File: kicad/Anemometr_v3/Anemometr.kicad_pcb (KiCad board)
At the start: 2 copper layers, 45 x 45 mm, 150 parts, among them J1 TxD, J10 +Z1, J11 +Z2, J12 +Z3, J13 +Z4, J14 -Z1, J15 -Z2, J16 -Z3, J17 -Z4, J18 1 TxD+, J19 2 TxD-, J2 RxD, J20 3 RxD+, J21 4-5, J22 6 RxD-, J23 7-8, J24 Conn_01x01_Female, J25 Conn_01x01_Female, J3 SCL, J4 SDA, J5 RST, J6 +EXT, J7 -EXT, J8 SWD, J9 SWC, Q1 5N10, U1 STM32F103C8Tx, U2 TS5A3166DBVR, U3 TS5A3166DBVR, U4 LMR14206, U6 NCP1117-3.3, U8 TLV3201DBV, U9 MCP1703-3.3, Y1 CSTCE8M00G52A-R0, Y2 ECS-250-20-33

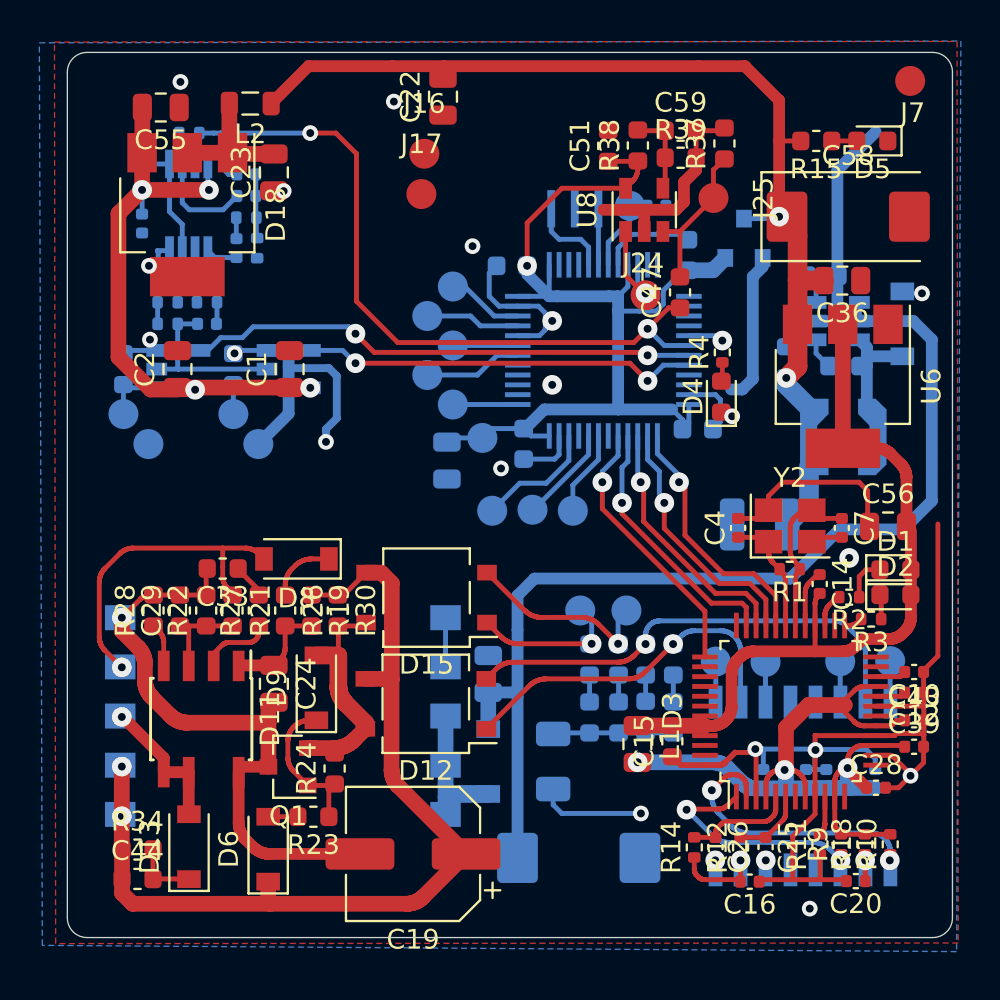
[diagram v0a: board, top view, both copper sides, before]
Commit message: изменено:      kicad/Anemometr_v3/Anemometr-cache.lib 	изменено:      kicad/Anemometr_v3/Anemometr.kicad_pcb 	изменено:      kicad/Anemometr_v3/Anemometr.kicad_pcb-bak 	изменено:      kicad/Anemometr_v3/Anemometr.sch 	изменено:      kicad/Anemometr_v3/Anemometr.sch-bak 	новый файл:    stm32cubeide/Anemometer/Debug/Core/Src/dhcp.d 	новый файл:    stm32cubeide/Anemometer/Debug/Core/Src/dhcp.o 	новый файл:    stm32cubeide/Anemometer/Debug/Core/Src/dhcp.su 	новый файл:    stm32cubeide/Anemometer/Debug/Core/Src/dns.d 	новый файл:    stm32cubeide/Anemometer/Debug/Core/Src/dns.o 	новый файл:    stm32cubeide/Anemometer/Debug/Core/Src/dns.su 	новый файл:    stm32cubeide/Anemometer/Debug/Core/Src/socket.d 	новый файл:    stm32cubeide/Anemometer/Debug/Core/Src/socket.o 	новый файл:    stm32cubeide/Anemometer/Debug/Core/Src/socket.su 	новый файл:    stm32cubeide/Anemometer/Debug/Core/Src/w5500.d 	новый файл:    stm32cubeide/Anemometer/Debug/Core/Src/w5500.o 	новый файл:    stm32cubeide/Anemometer/Debug/Core/Src/w5500.su 	новый файл:    stm32cubeide/Anemometer/Debug/Core/Src/wizchip_conf.d 	новый файл:    stm32cubeide/Anemometer/Debug/Core/Src/wizchip_conf.o 	новый файл:    stm32cubeide/Anemometer/Debug/Core/Src/wizchip_conf.su 	новый файл:    stm32cubeide/Anemometer/Debug/Drivers/STM32F1xx_HAL_Driver/Src/stm32f1xx_hal_i2c.d 	новый файл:    stm32cubeide/Anemometer/Debug/Drivers/STM32F1xx_HAL_Driver/Src/stm32f1xx_hal_i2c.o 	новый файл:    stm32cubeide/Anemometer/Debug/Drivers/STM32F1xx_HAL_Driver/Src/stm32f1xx_hal_i2c.su 	новый файл:    stm32cubeide/Anemometer/Drivers/STM32F1xx_HAL_Driver/Inc/stm32f1xx_hal_iwdg.h 	новый файл:    stm32cubeide/Anemometer/Drivers/STM32F1xx_HAL_Driver/Inc/stm32f1xx_hal_spi.h 	новый файл:    stm32cubeide/Anemometer/Drivers/STM32F1xx_HAL_Driver/Src/stm32f1xx_hal_iwdg.c 	новый файл:    stm32cubeide/Anemometer/Drivers/STM32F1xx_HAL_Driver/Src/stm32f1xx_hal_spi.c 	новый файл:    stm32cubeide/Anemometer/Release/Anemometer.hex 	новый файл:    stm32cubeide/A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
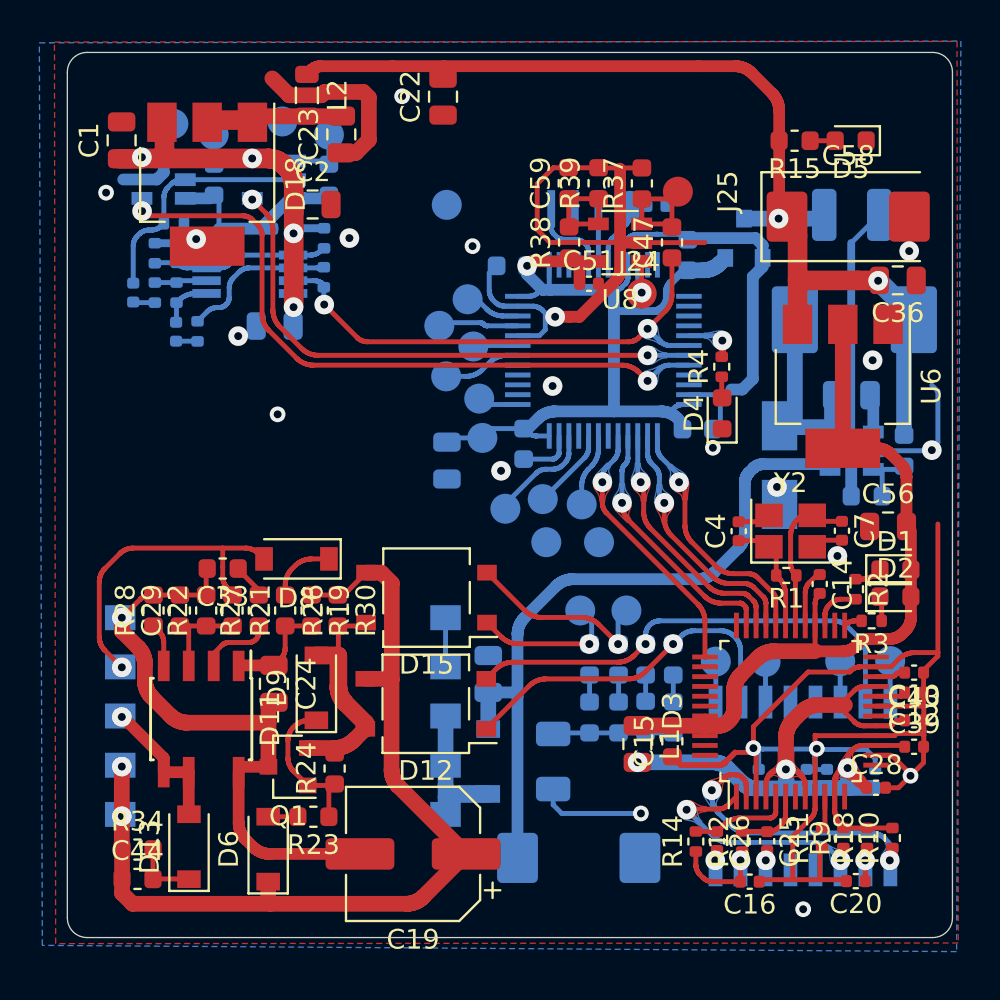
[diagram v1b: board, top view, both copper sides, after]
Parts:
- removed C40, C41: 390p, Capacitor_SMD:C_0402_1005Metric
- removed R31: 1.3k, Resistor_SMD:R_0402_1005Metric
- C51: footprint Capacitor_SMD:C_0603_1608Metric -> Capacitor_SMD:C_0402_1005Metric
- C53: footprint Capacitor_SMD:C_0603_1608Metric -> Capacitor_SMD:C_0805_2012Metric
- C55, J16, J17, J7: moved to B.Cu
- D13, D8: value MBR0540 -> F7
- D16: value MBR0540 -> SS34
- D17: value MBR0540 -> SS56; footprint Diode_SMD:D_SOD-123 -> Diode_SMD:D_SMA
- L5: value CoilCraft HLPS4018-472MR -> 15uH; footprint Inductor_SMD:L_Coilcraft_LPS4018 -> Inductor_SMD:L_Abracon_ASPI-0630LR
- R17: value 110k -> 100k
- moved J7 29.9 mm to (43.4, 84.9)
- moved J16 21.7 mm to (46.0, 84.9)
- moved J15 17.8 mm to (29.9, 63.5), turned to 180 degrees
- moved J10 17.6 mm to (32.3, 64.2), turned to 180 degrees
- moved J14 16.8 mm to (24.4, 63.6), turned to 180 degrees
- moved C54 16.4 mm to (58.9, 68.3), turned to 180 degrees
- moved C1 14.4 mm to (21.8, 64.5)
- moved J11 14.2 mm to (26.4, 64.2), turned to 180 degrees
- moved R5 14.2 mm to (32.3, 66.5), turned to 90 degrees
- moved C55 12.5 mm to (29.5, 73.9), turned to 0 degrees
- moved U3 11.5 mm to (23.9, 66.5), turned to 180 degrees
- moved R41 11.4 mm to (59.6, 82.6), turned to 180 degrees
- moved C2 10.8 mm to (31.5, 67.7), turned to 0 degrees
- moved U2 10.8 mm to (29.5, 66.5), turned to 180 degrees
- moved R33 10.0 mm to (32.0, 71.4), turned to 270 degrees
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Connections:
- net Net-(C22-Pad2) renamed /5.6-6v
- net Net-(C3-Pad2) renamed /Rst
- net Net-(J1-Pad1) renamed /TxD
- net Net-(J10-Pad1) renamed /+Z1
- net Net-(J11-Pad1) renamed /+Z2
- net Net-(J12-Pad1) renamed /+Z3
- net Net-(J13-Pad1) renamed /+Z4
- net Net-(J2-Pad1) renamed /RxD
- net Net-(J3-Pad1) renamed /SCL
- net Net-(J4-Pad1) renamed /SDA
- net Net-(J8-Pad1) renamed /SWD
- net Net-(J9-Pad1) renamed /SWC
- D3 pad 23: (no net) -> GND
- D7 pad 6: Net-(C41-Pad2) -> Net-(D7-Pad6)
- R29 pad 1: Net-(C40-Pad1) -> Net-(D7-Pad6)
- R33 pad 1: Net-(C41-Pad2) -> Net-(D7-Pad6)
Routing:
- net GND: track 146.0 -> 190.4 mm, vias 19 -> 21
- net /12-16v: track 53.5 -> 37.7 mm
- net Z2: track 20.2 -> 34.9 mm
- net Analog: track 40.8 -> 26.5 mm
- net +5VA: track 30.5 -> 21.4 mm
- net Net-(D7-Pad6): track 0.00 -> 8.04 mm
- net +3V3: track 50.5 -> 43.3 mm
- net Net-(C41-Pad2): track 6.82 -> 0.00 mm
- net Net-(C18-Pad2): track 8.93 -> 12.5 mm
- net Net-(C40-Pad1): track 3.27 -> 0.00 mm
- net /5.6-6v: track 57.4 -> 54.4 mm
- net Z1: track 26.0 -> 28.3 mm
- net SensorInput: track 5.28 -> 3.13 mm
- net Net-(R41-Pad1): track 4.97 -> 3.00 mm
- net Net-(C59-Pad1): track 4.37 -> 5.80 mm
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
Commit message: изменено:      kicad/Anemometr_v3/Anemometr-cache.lib 	изменено:      kicad/Anemometr_v3/Anemometr.kicad_pcb 	изменено:      kicad/Anemometr_v3/Anemometr.kicad_pcb-bak 	изменено:      kicad/Anemometr_v3/Anemometr.pro 	изменено:      kicad/Anemometr_v3/Anemometr.sch 	изменено:      kicad/Anemometr_v3/Anemometr.sch-bak 	изменено:      kicad/Anemometr_v3/fp-info-cache
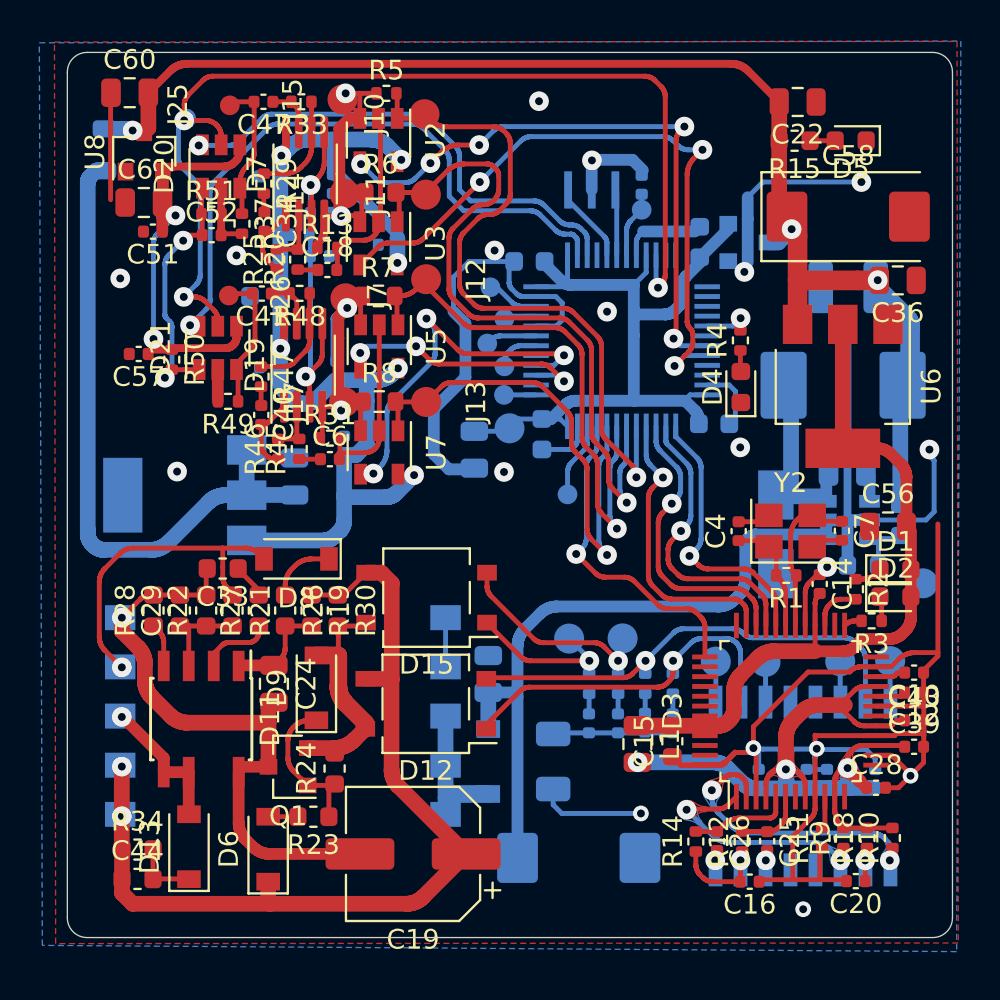
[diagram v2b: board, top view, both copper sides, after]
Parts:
- removed R38: 100k, Resistor_SMD:R_0603_1608Metric
- removed R39: 3k, Resistor_SMD:R_0603_1608Metric
- added C32: 0.1uF, Capacitor_SMD:C_0402_1005Metric, B.Cu at (29.2, 66.3)
- added C40: 100nF, Capacitor_SMD:C_0402_1005Metric, F.Cu at (28.9, 78.4)
- added C41: 1,5nF, Capacitor_SMD:C_0402_1005Metric, F.Cu at (28.9, 72.3)
- added C5: 0.1uF, Capacitor_SMD:C_0402_1005Metric, B.Cu at (33.1, 80.0)
- added C52: 0.1uF, Capacitor_SMD:C_0402_1005Metric, F.Cu at (26.3, 69.3)
- added C57: 0.1uF, Capacitor_SMD:C_0402_1005Metric, F.Cu at (22.6, 75.3)
- added C6: 10nF, Capacitor_SMD:C_0402_1005Metric, F.Cu at (32.4, 80.7)
- added C60: 10uF, Capacitor_SMD:C_0805_2012Metric, F.Cu at (22.2, 62.0)
- added C61: 10uF, Capacitor_SMD:C_0805_2012Metric, F.Cu at (22.9, 67.6)
- added D19: MAX4477, Package_SO:MSOP-8_3x3mm_P0.65mm, F.Cu at (31.0, 75.9)
- added D20: TLV3501, Package_TO_SOT_SMD:SOT-23-6, F.Cu at (26.8, 65.8)
- added D21: TLV3501, Package_TO_SOT_SMD:SOT-23-6, F.Cu at (26.6, 75.0)
- added J26: Conn_01x01_Female, My-library:ConnMini, F.Cu at (27.2, 72.4)
- added R31: 20k, Resistor_SMD:R_0402_1005Metric, F.Cu at (32.4, 79.6)
- added R45: 1k, Resistor_SMD:R_0402_1005Metric, F.Cu at (30.8, 80.2)
- added R46: 100k, Resistor_SMD:R_0402_1005Metric, F.Cu at (29.7, 80.2)
- added R47: 5.1k, Resistor_SMD:R_0402_1005Metric, F.Cu at (28.9, 76.5)
- added R48: 100k, Resistor_SMD:R_0402_1005Metric, F.Cu at (30.8, 72.2)
- added R49: 10k, Resistor_SMD:R_0402_1005Metric, F.Cu at (27.2, 77.7)
- added R50: 100k, Resistor_SMD:R_0402_1005Metric, F.Cu at (24.3, 75.6)
- added R51: 3k, Resistor_SMD:R_0402_1005Metric, F.Cu at (26.3, 68.2)
- added R7: 3k, Resistor_SMD:R_0603_1608Metric, F.Cu at (34.8, 72.4)
- added R8: 3k, Resistor_SMD:R_0603_1608Metric, F.Cu at (34.9, 77.8)
- added U5: TS5A3166DBVR, Package_TO_SOT_SMD:SOT-23-5, F.Cu at (34.9, 75.0)
- added U7: TS5A3166DBVR, Package_TO_SOT_SMD:SOT-23-5, F.Cu at (34.9, 80.3)
- C1, C2: footprint Capacitor_SMD:C_0805_2012Metric -> Capacitor_SMD:C_0402_1005Metric; moved to B.Cu
- C18, C34, D7, J10, J11, J12, J13, J14, J15, J17, J7, R13, R20, R29, R33, R6, U2, U3: moved to F.Cu
- C23, D18, L2: moved to B.Cu
- C42, C45, C46, C47, C48: footprint Capacitor_SMD:C_0603_1608Metric -> Capacitor_SMD:C_0402_1005Metric
- C55: footprint Capacitor_SMD:C_0805_2012Metric -> Capacitor_SMD:C_0603_1608Metric
- C59: footprint Capacitor_SMD:C_0603_1608Metric -> Capacitor_SMD:C_0402_1005Metric; moved to B.Cu
- J1, J2, J25, J3, J4, J5, J8, J9: footprint My-library:SMD-CONN -> My-library:ConnMini
- J24: footprint My-library:SMD-CONN -> My-library:ConnMini; moved to B.Cu
- R17: value 100k -> 110k
- R21: value 30k -> 43k
- R25: value 300k -> 100k; moved to F.Cu
- R32, R35, R36, R37, R40: footprint Resistor_SMD:R_0603_1608Metric -> Resistor_SMD:R_0402_1005Metric
- R5: footprint Resistor_SMD:R_0603_1608Metric -> Resistor_SMD:R_0402_1005Metric; moved to F.Cu
- U8: value TLV3201DBV -> MCP1703-3.3; footprint Package_TO_SOT_SMD:SOT-23-5 -> Package_TO_SOT_SMD:SOT-23
- moved J24 24.8 mm to (25.0, 63.4)
- moved U8 24.6 mm to (22.9, 65.1), turned to 90 degrees
- moved J25 23.2 mm to (27.3, 62.7), turned to 270 degrees
- moved C51 22.3 mm to (23.4, 69.1), turned to 180 degrees
- moved C47 22.0 mm to (29.0, 62.5), turned to 180 degrees
- moved R37 20.4 mm to (27.9, 68.7), turned to 270 degrees
- moved C22 18.0 mm to (56.1, 62.5), turned to 180 degrees
- moved C59 17.9 mm to (29.2, 76.0), turned to 180 degrees
- moved C23 17.6 mm to (30.6, 81.6), turned to 270 degrees
- moved J16 16.6 mm to (62.5, 87.0)
- moved J7 16.1 mm to (33.1, 72.5), turned to 90 degrees
- moved C1 16.0 mm to (32.7, 76.2)
- moved D18 15.9 mm to (25.0, 82.5), turned to 180 degrees
- moved J12 13.9 mm to (37.2, 71.5), turned to 90 degrees
- moved U3 11.4 mm to (34.8, 69.7), turned to 270 degrees
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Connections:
- net /SWC renamed /swc
- net /SWD renamed /swd
- net Net-(C21-Pad2) renamed a
- C47 pad 1: Analog -> Net-(C47-Pad1)
- C51 pad 1: +3V3 -> +3.3VP
- C59 pad 1: Net-(C59-Pad1) -> +5VA
- D7 pad 7: Analog -> Net-(C47-Pad1)
- J24 pad 1: SensorInput -> SInput
- R33 pad 2: Analog -> Net-(C47-Pad1)
- U1 pad 10: SensorInput -> SInput
- U1 pad 18: Analog -> (no net)
- U1 pad 2: (no net) -> Z3-4
- U1 pad 29: nrst -> /+Z1
- U1 pad 3: (no net) -> Z1-2
- U1 pad 30: (no net) -> /+Z2
- U1 pad 33: (no net) -> nrst
- U1 pad 39: (no net) -> Z3
- U1 pad 40: (no net) -> Z4
- U8 pad 1: SensorInput -> GND
- U8 pad 2: GND -> +3.3VP
- U8 pad 3: Net-(C47-Pad2) -> /5.6-6v
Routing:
- net SInput: track 0.00 -> 53.4 mm, vias 0 -> 3
- net +5VA: track 21.4 -> 54.4 mm, vias 4 -> 6
- net /+Z2: track 3.04 -> 35.9 mm, vias 0 -> 1
- net Z3-4: track 0.00 -> 32.2 mm, vias 0 -> 1
- net /+Z1: track 3.26 -> 35.0 mm, vias 0 -> 1
- net Net-(C23-Pad2): track 6.86 -> 33.4 mm
- net Analog: track 26.5 -> 0.00 mm, vias 2 -> 0
- net Z1-2: track 0.00 -> 24.9 mm, vias 0 -> 1
- net /+Z3: track 3.73 -> 28.1 mm, vias 0 -> 1
- net /+Z4: track 4.16 -> 25.9 mm, vias 0 -> 1
- net +3.3VP: track 0.00 -> 21.4 mm, vias 0 -> 2
- net Z4: track 0.00 -> 19.2 mm, vias 0 -> 3
- net Z3: track 0.00 -> 13.5 mm, vias 0 -> 3
- net Net-(C52-Pad1): track 0.00 -> 13.2 mm, vias 0 -> 2
- net /5.6-6v: track 54.4 -> 67.2 mm, vias 2 -> 3
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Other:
- net class Default: via_dia 0.8 -> 1
